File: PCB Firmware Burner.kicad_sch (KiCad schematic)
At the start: 22 parts, among them J2 Conn_01x07_Male, Q1 BSS138, Q2 BSS138, T5V0b1 T5V0b1, T5V0b2 T5V0b2, T5V0c1 T5V0c1, T5V0c2 T5V0c2

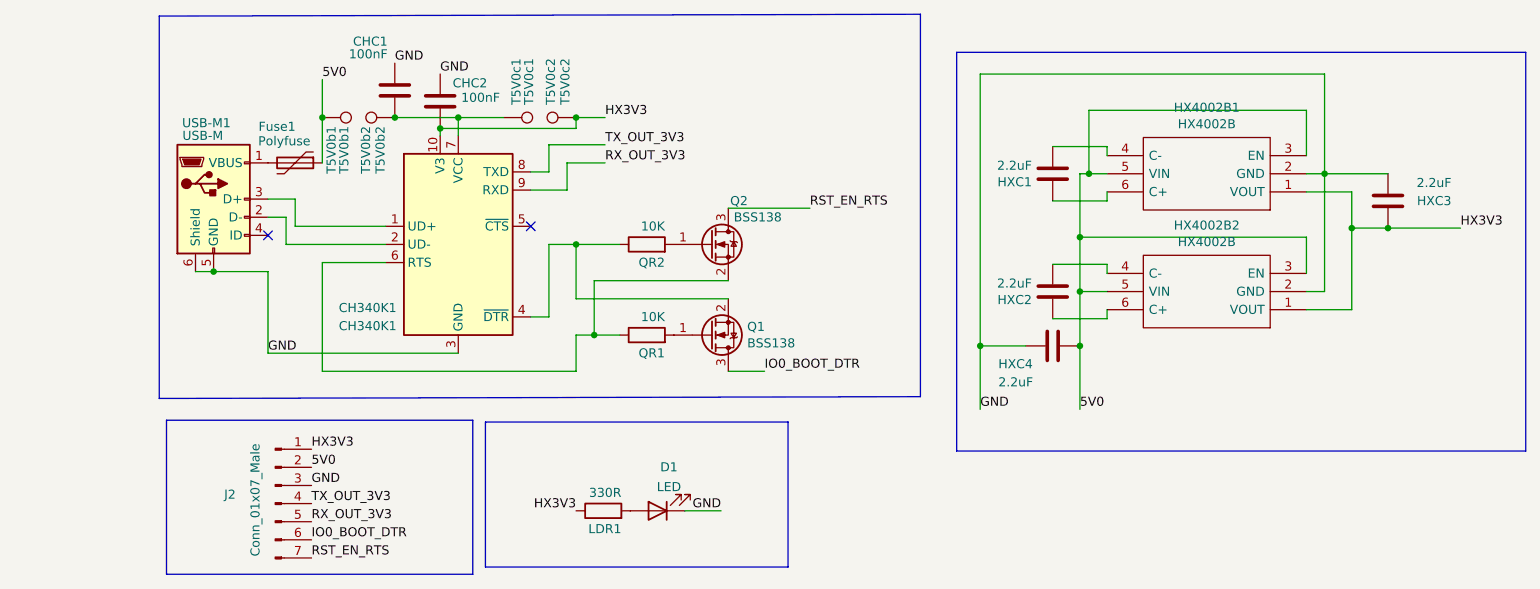
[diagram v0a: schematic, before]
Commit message: rev 1.4
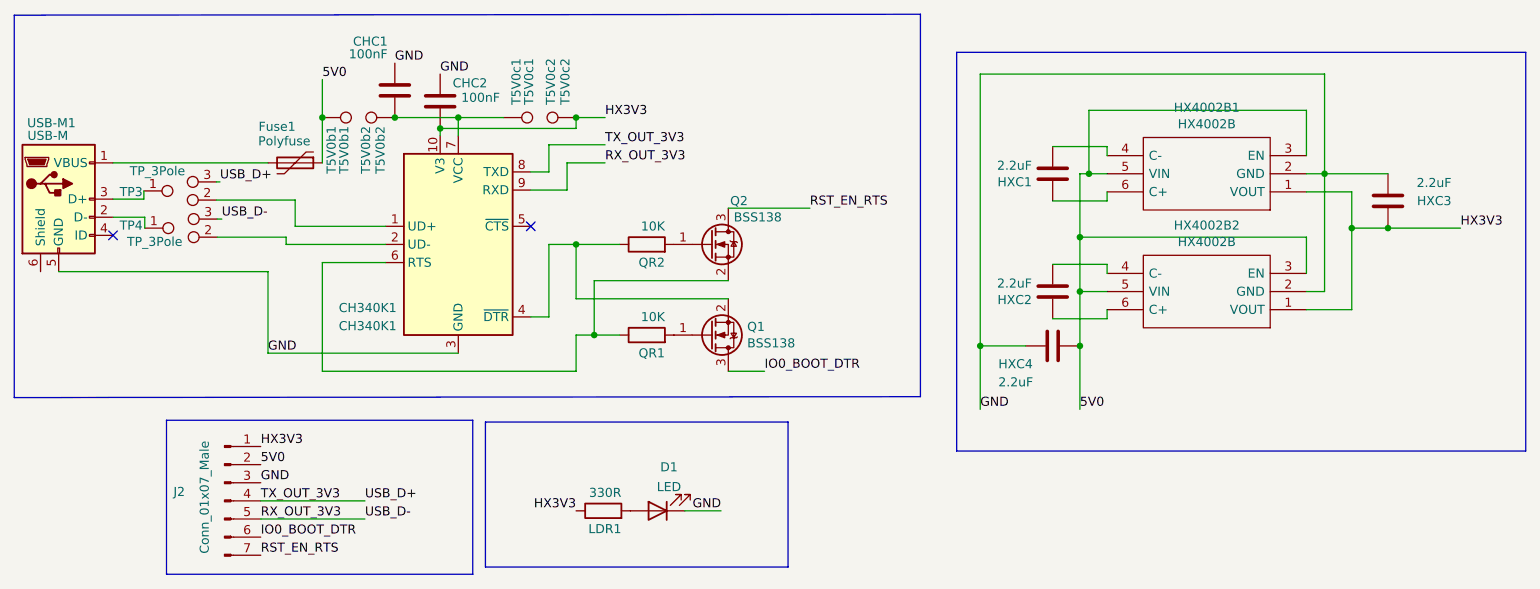
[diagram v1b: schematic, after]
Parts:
- added TP3, TP4: TP_3Pole, TestPoint:TestPoint_Pad_1.5mm 3 points, symbol Connector:TestPoint_3Pole
- J2: footprint TerminalBlock_Phoenix:TerminalBlock_Phoenix_MPT-0,5-7-2.54_1x07_P2.54mm_Horizontal -> Connector_PinHeader_2.54mm:PinHeader_1x07_P2.54mm_Horizontal
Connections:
- net GND: no longer USB-M1.6 (Shield)
- net RX_OUT_3V3: now also TP4.3
- net TX_OUT_3V3: now also TP3.3
- net at CH340K1.1 (UD+): now also TP3.2; no longer USB-M1.3 (D+)
- net at CH340K1.2 (UD-): now also TP4.2; no longer USB-M1.2 (D-)
- new net: TP4.1, USB-M1.2 (D-)
- new net: TP3.1, USB-M1.3 (D+)
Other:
- moved on the sheet: J2, USB-M1

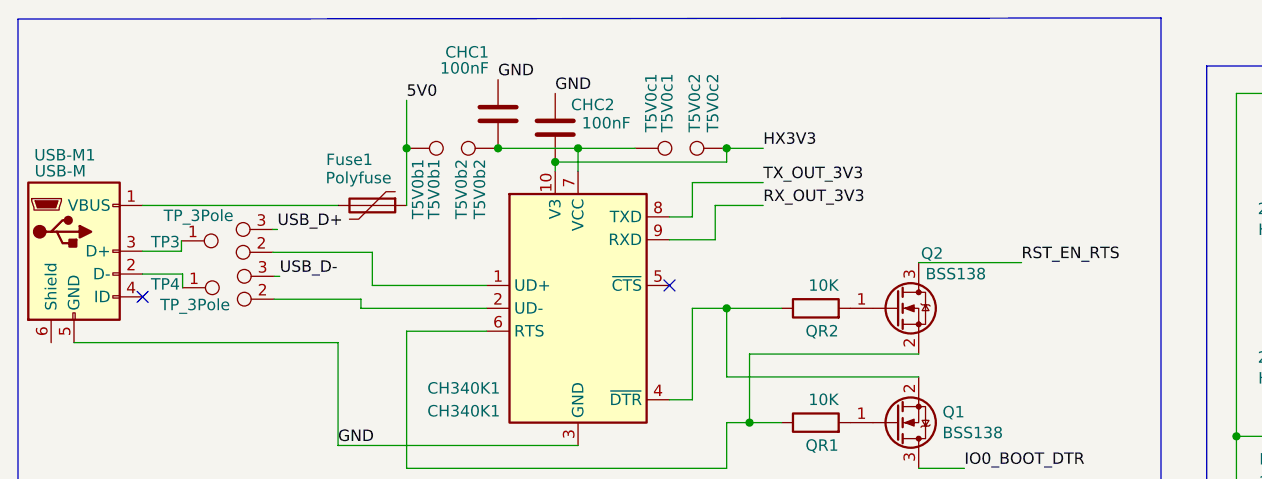
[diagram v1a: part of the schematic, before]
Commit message: update
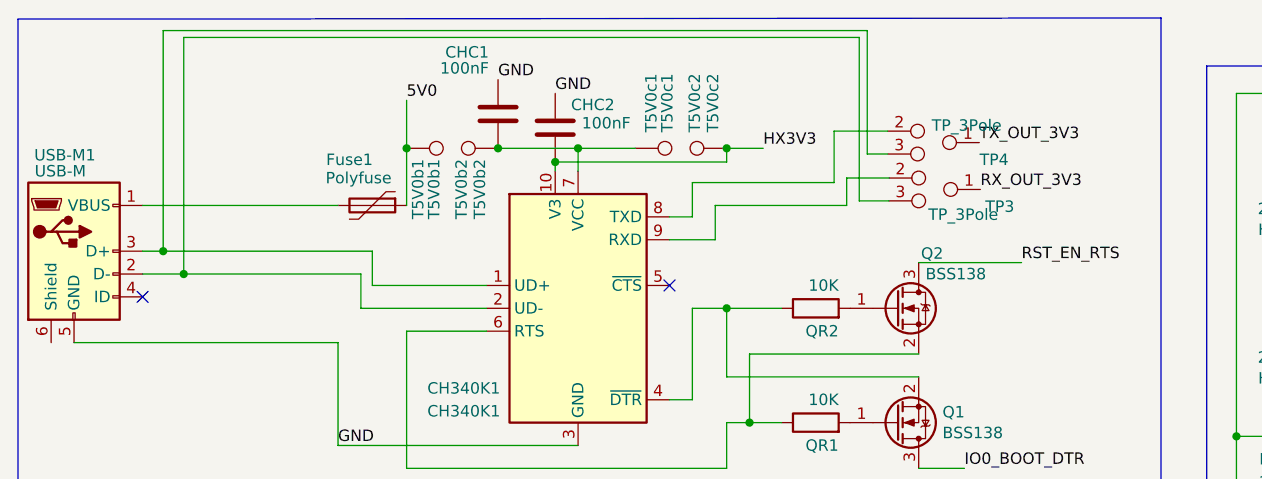
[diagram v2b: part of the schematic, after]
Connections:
- net RX_OUT_3V3: now also TP3.1; no longer CH340K1.9 (RXD), TP4.3
- net TX_OUT_3V3: now also TP4.1; no longer CH340K1.8 (TXD), TP3.3
- net at CH340K1.1 (UD+): now also TP4.3, USB-M1.3 (D+); no longer TP3.2
- net at CH340K1.2 (UD-): now also TP3.3, USB-M1.2 (D-); no longer TP4.2
- new net: CH340K1.8 (TXD), TP4.2
- new net: CH340K1.9 (RXD), TP3.2
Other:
- moved on the sheet: TP3, TP4
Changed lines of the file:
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@@
   (junction (at 182.88 74.93) (diameter 0) (color 0 0 0 0)
   )
+  (junction (at 50.673 81.026) (diameter 0) (color 0 0 0 0)
+  )
   (junction (at 219.71 82.55) (diameter 0) (color 0 0 0 0)
+  )
+  (junction (at 48.387 78.486) (diameter 0) (color 0 0 0 0)
   )
   (junction (at 110.998 84.836) (diameter 0) (color 0 0 0 0)
@@
     (stroke (width 0) (type default) (color 0 0 0 0))
   )
+  (wire (pts (xy 50.673 81.026) (xy 70.358 81.026))
+    (stroke (width 0) (type default) (color 0 0 0 0))
+  )
   (polyline (pts (xy 98.298 109.728) (xy 98.298 130.048))
     (stroke (width 0) (type default) (color 0 0 0 0))
   )
-  (wire (pts (xy 61.087 76.073) (xy 60.579 76.073))
-    (stroke (width 0) (type default) (color 0 0 0 0))
-  )
   (wire (pts (xy 75.438 61.722) (xy 75.438 67.056))
     (stroke (width 0) (type default) (color 0 0 0 0))
   )
+  (wire (pts (xy 122.936 65.151) (xy 128.905 65.151))
+    (stroke (width 0) (type default) (color 0 0 0 0))
+  )
   (wire (pts (xy 67.818 88.646) (xy 67.818 100.076))
     (stroke (width 0) (type default) (color 0 0 0 0))
   )
-  (wire (pts (xy 60.579 78.613) (xy 71.628 78.613))
-    (stroke (width 0) (type default) (color 0 0 0 0))
-  )
   (wire (pts (xy 181.61 91.44) (xy 181.61 99.06))
     (stroke (width 0) (type default) (color 0 0 0 0))
   )
-  (wire (pts (xy 70.358 83.82) (xy 70.358 84.836))
+  (wire (pts (xy 70.358 81.026) (xy 70.358 84.836))
     (stroke (width 0) (type default) (color 0 0 0 0))
   )
@@
     (stroke (width 0) (type default) (color 0 0 0 0))
   )
+  (wire (pts (xy 48.387 53.975) (xy 48.387 78.486))
+    (stroke (width 0) (type default) (color 0 0 0 0))
+  )
   (polyline (pts (xy 32.258 52.705) (xy 159.258 52.578))
     (stroke (width 0) (type default) (color 0 0 0 0))
@@
     (stroke (width 0) (type default) (color 0 0 0 0))
   )
-  (wire (pts (xy 109.728 73.406) (xy 115.062 73.406))
+  (wire (pts (xy 109.728 73.406) (xy 124.333 73.406))
     (stroke (width 0) (type default) (color 0 0 0 0))
   )
@@
     (stroke (width 0) (type default) (color 0 0 0 0))
   )
+  (wire (pts (xy 125.73 54.737) (xy 50.673 54.737))
+    (stroke (width 0) (type default) (color 0 0 0 0))
+  )
   (wire (pts (xy 110.998 97.536) (xy 113.538 97.536))
     (stroke (width 0) (type default) (color 0 0 0 0))
@@
     (stroke (width 0) (type default) (color 0 0 0 0))
   )
-  (wire (pts (xy 107.188 70.866) (xy 115.062 70.866))
+  (wire (pts (xy 107.188 70.866) (xy 122.936 70.866))
     (stroke (width 0) (type default) (color 0 0 0 0))
   )
@@
     (stroke (width 0) (type default) (color 0 0 0 0))
   )
+  (wire (pts (xy 129.032 72.898) (xy 125.73 72.898))
+    (stroke (width 0) (type default) (color 0 0 0 0))
+  )
   (wire (pts (xy 110.998 67.056) (xy 110.998 68.58))
     (stroke (width 0) (type default) (color 0 0 0 0))
@@
     (stroke (width 0) (type default) (color 0 0 0 0))
   )
+  (wire (pts (xy 48.387 78.486) (xy 71.628 78.486))
+    (stroke (width 0) (type default) (color 0 0 0 0))
+  )
   (wire (pts (xy 213.36 74.93) (xy 215.9 74.93))
     (stroke (width 0) (type default) (color 0 0 0 0))
   )
-  (wire (pts (xy 71.628 78.613) (xy 71.628 82.296))
+  (wire (pts (xy 71.628 78.486) (xy 71.628 82.296))
+    (stroke (width 0) (type default) (color 0 0 0 0))
+  )
+  (wire (pts (xy 126.619 67.691) (xy 126.619 53.975))
     (stroke (width 0) (type default) (color 0 0 0 0))
   )
@@
     (stroke (width 0) (type default) (color 0 0 0 0))
   )
-  (wire (pts (xy 50.419 78.486) (xy 50.419 77.343))
+  (wire (pts (xy 126.619 53.975) (xy 48.387 53.975))
     (stroke (width 0) (type default) (color 0 0 0 0))
   )
@@
     (stroke (width 0) (type default) (color 0 0 0 0))
   )
+  (wire (pts (xy 128.905 67.691) (xy 126.619 67.691))
+    (stroke (width 0) (type default) (color 0 0 0 0))
+  )
+  (wire (pts (xy 124.333 70.358) (xy 124.333 73.406))
+    (stroke (width 0) (type default) (color 0 0 0 0))
+  )
   (wire (pts (xy 181.61 91.44) (xy 181.61 83.82))
     (stroke (width 0) (type default) (color 0 0 0 0))
@@
     (stroke (width 0) (type default) (color 0 0 0 0))
   )
-  (wire (pts (xy 50.546 81.026) (xy 50.546 82.55))
-    (stroke (width 0) (type default) (color 0 0 0 0))
-  )
   (wire (pts (xy 110.998 67.056) (xy 115.062 67.056))
     (stroke (width 0) (type default) (color 0 0 0 0))
   )
-  (wire (pts (xy 46.101 81.026) (xy 50.546 81.026))
+  (wire (pts (xy 46.101 81.026) (xy 50.673 81.026))
     (stroke (width 0) (type default) (color 0 0 0 0))
   )
@@
     (stroke (width 0) (type default) (color 0 0 0 0))
   )
-  (wire (pts (xy 61.341 81.28) (xy 60.706 81.28))
-    (stroke (width 0) (type default) (color 0 0 0 0))
-  )
   (polyline (pts (xy 164.338 113.792) (xy 244.094 113.792))
     (stroke (width 0) (type default) (color 0 0 0 0))
@@
     (stroke (width 0) (type default) (color 0 0 0 0))
   )
+  (wire (pts (xy 122.936 70.866) (xy 122.936 65.151))
+    (stroke (width 0) (type default) (color 0 0 0 0))
+  )
   (wire (pts (xy 38.481 88.646) (xy 67.818 88.646))
     (stroke (width 0) (type default) (color 0 0 0 0))
@@
     (stroke (width 0) (type default) (color 0 0 0 0))
   )
+  (wire (pts (xy 125.73 72.898) (xy 125.73 54.737))
+    (stroke (width 0) (type default) (color 0 0 0 0))
+  )
   (wire (pts (xy 219.71 77.47) (xy 219.71 82.55))
     (stroke (width 0) (type default) (color 0 0 0 0))
@@
     (stroke (width 0) (type default) (color 0 0 0 0))
   )
-  (wire (pts (xy 46.101 78.486) (xy 50.419 78.486))
-    (stroke (width 0) (type default) (color 0 0 0 0))
-  )
   (polyline (pts (xy 96.52 131.064) (xy 96.52 109.474))
     (stroke (width 0) (type default) (color 0 0 0 0))
@@
     (stroke (width 0) (type default) (color 0 0 0 0))
   )
+  (wire (pts (xy 50.673 54.737) (xy 50.673 81.026))
+    (stroke (width 0) (type default) (color 0 0 0 0))
+  )
   (polyline (pts (xy 140.716 130.048) (xy 140.716 109.728))
     (stroke (width 0) (type default) (color 0 0 0 0))
@@
     (stroke (width 0) (type default) (color 0 0 0 0))
   )
-  (wire (pts (xy 60.706 83.82) (xy 70.358 83.82))
-    (stroke (width 0) (type default) (color 0 0 0 0))
-  )
   (wire (pts (xy 182.88 74.93) (xy 185.42 74.93))
     (stroke (width 0) (type default) (color 0 0 0 0))
@@
     (stroke (width 0) (type default) (color 0 0 0 0))
   )
+  (wire (pts (xy 46.101 78.486) (xy 48.387 78.486))
+    (stroke (width 0) (type default) (color 0 0 0 0))
+  )
   (wire (pts (xy 75.438 67.056) (xy 75.438 73.406))
     (stroke (width 0) (type default) (color 0 0 0 0))
   )
   (wire (pts (xy 91.948 68.58) (xy 110.998 68.58))
+    (stroke (width 0) (type default) (color 0 0 0 0))
+  )
+  (wire (pts (xy 129.032 70.358) (xy 124.333 70.358))
     (stroke (width 0) (type default) (color 0 0 0 0))
   )
@@
     (effects (font (size 1.27 1.27)) (justify left bottom))
   )
-  (label "USB_D+" (at 61.087 76.073 0)
-    (effects (font (size 1.27 1.27)) (justify left bottom))
-  )
-  (label "RX_OUT_3V3" (at 115.062 73.406 0)
+  (label "RX_OUT_3V3" (at 139.192 71.628 0)
     (effects (font (size 1.27 1.27)) (justify left bottom))
   )
@@
     (effects (font (size 1.27 1.27)) (justify right bottom))
   )
-  (label "TX_OUT_3V3" (at 115.062 70.866 0)
+  (label "TX_OUT_3V3" (at 139.065 66.421 0)
     (effects (font (size 1.27 1.27)) (justify left bottom))
   )
@@
   )
   (label "TX_OUT_3V3" (at 66.802 120.777 0)
-    (effects (font (size 1.27 1.27)) (justify left bottom))
-  )
-  (label "USB_D-" (at 61.341 81.28 0)
     (effects (font (size 1.27 1.27)) (justify left bottom))
   )
@@
     (pin "1")
   )
-  (symbol (lib_id "Connector:TestPoint_3Pole") (at 55.499 78.613 0) (unit 1)
-    (in_bom yes) (on_board yes)
-    (property "Reference" "TP3" (id 0) (at 48.641 77.47 0))
-    (property "Value" "TP_3Pole" (id 1) (at 52.324 74.549 0))
-    (property "Footprint" "TestPoint:TestPoint_Pad_1.5mm 3 points" (id 2) (at 55.499 78.613 0)
-      (effects (font (size 1.27 1.27)) hide)
-    )
-    (property "Datasheet" "~" (id 3) (at 55.753 77.343 0)
+  (symbol (lib_id "Connector:TestPoint_3Pole") (at 134.112 70.358 180) (unit 1)
+    (in_bom yes) (on_board yes)
+    (property "Reference" "TP3" (id 0) (at 141.351 73.533 0))
+    (property "Value" "TP_3Pole" (id 1) (at 137.287 74.422 0))
+    (property "Footprint" "TestPoint:TestPoint_Pad_1.5mm 3 points" (id 2) (at 134.112 70.358 0)
+      (effects (font (size 1.27 1.27)) hide)
+    )
+    (property "Datasheet" "~" (id 3) (at 133.858 71.628 0)
       (effects (font (size 1.27 1.27)) hide)
     )
@@
     (pin "1")
   )
-  (symbol (lib_id "Connector:TestPoint_3Pole") (at 55.626 83.82 0) (unit 1)
-    (in_bom yes) (on_board yes)
-    (property "Reference" "TP4" (id 0) (at 48.641 82.169 0))
-    (property "Value" "TP_3Pole" (id 1) (at 51.943 84.455 0))
-    (property "Footprint" "TestPoint:TestPoint_Pad_1.5mm 3 points" (id 2) (at 55.626 83.82 0)
-      (effects (font (size 1.27 1.27)) hide)
-    )
-    (property "Datasheet" "~" (id 3) (at 55.88 82.55 0)
-      (effects (font (size 1.27 1.27)) hide)
-    )
+  (symbol (lib_id "Connector:TestPoint_3Pole") (at 133.985 65.151 180) (unit 1)
+    (in_bom yes) (on_board yes)
+    (property "Reference" "TP4" (id 0) (at 140.716 68.326 0))
+    (property "Value" "TP_3Pole" (id 1) (at 137.668 64.516 0))
+    (property "Footprint" "TestPoint:TestPoint_Pad_1.5mm 3 points" (id 2) (at 133.985 65.151 0)
+      (effects (font (size 1.27 1.27)) hide)
+    )
+    (property "Datasheet" "~" (id 3) (at 133.731 66.421 0)
+      (effects (font (size 1.27 1.27)) hide)
+    )
